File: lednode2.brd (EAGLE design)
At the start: 99.8 x 49.8 mm, 50 parts, among them Q1 AO3402, Q2 AO3402, Q3 AO3402, Q4 AO3402, Q5 AO3402

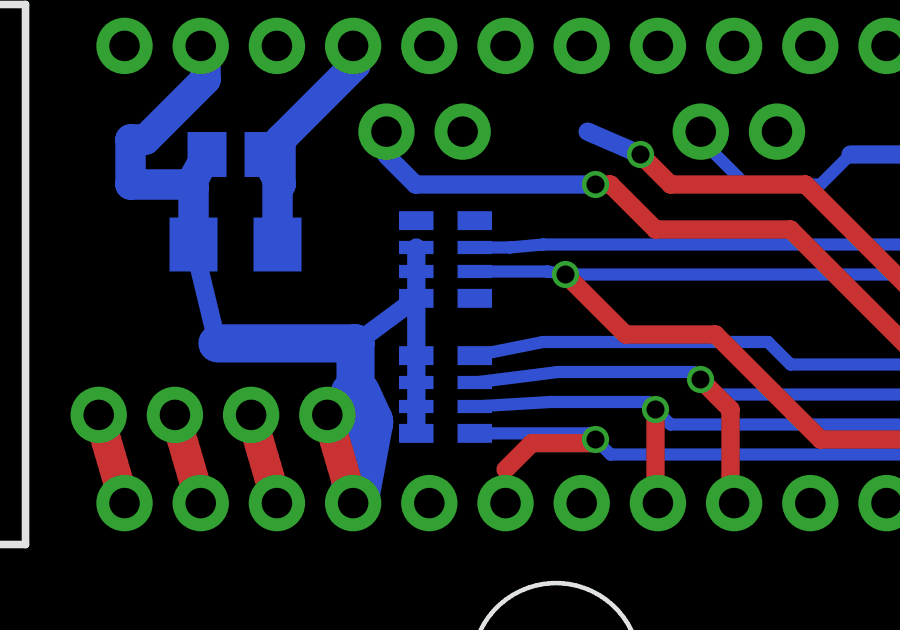
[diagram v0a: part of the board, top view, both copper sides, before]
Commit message: tuning.
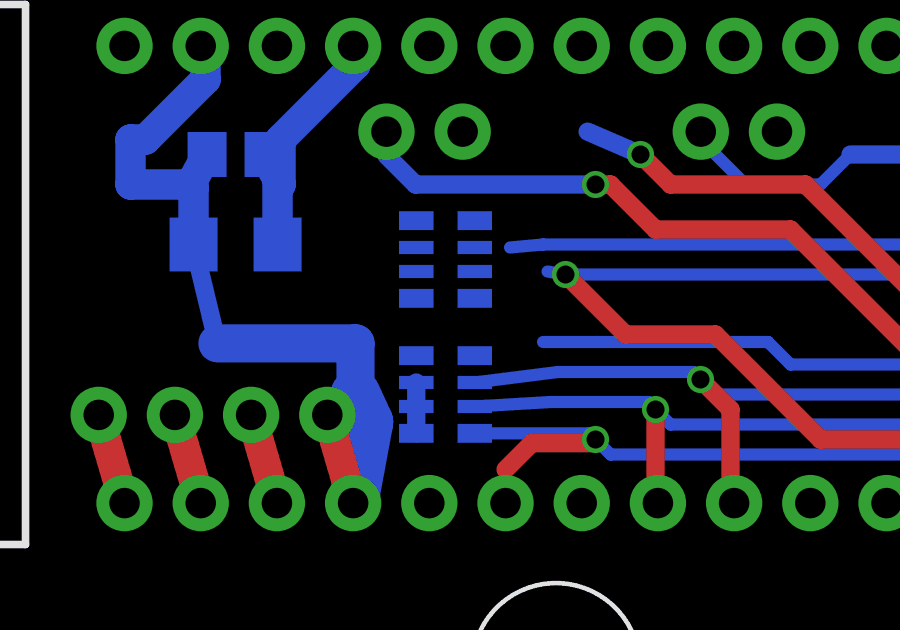
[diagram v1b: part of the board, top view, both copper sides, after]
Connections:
- new net N$12: RN4.3, RN4.4
- new net N$17: RN4.6, RN4.7
- net GND: no longer RN4.3, RN4.4
- net N$13: no longer RN2.5
- net SENSOR1: no longer RN4.8
- net SPOTLIGHT4: now also RN2.5; no longer RN4.7
- net SPOTLIGHT5: now also RN4.8; no longer RN4.6
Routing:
- net GND: track 36.4 -> 29.4 mm
- net SPOTLIGHT4: track 35.5 -> 33.1 mm
- net N$13: track 26.4 -> 24.1 mm
- net SPOTLIGHT5: track 19.6 -> 18.4 mm
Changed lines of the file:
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@@
 <contactref element="LEDS5" pad="3"/>
 <contactref element="Q5" pad="2"/>
-<contactref element="RN4" pad="3"/>
-<contactref element="RN4" pad="2"/>
-<contactref element="RN4" pad="1"/>
-<contactref element="RN2" pad="4"/>
-<wire x1="39.025" y1="28.9" x2="39.025" y2="28.1" width="0.6096" layer="16"/>
-<wire x1="39.025" y1="28.1" x2="39.025" y2="27.205" width="0.6096" layer="16"/>
 <wire x1="39.025" y1="22.705" x2="39.025" y2="23.6" width="0.6096" layer="16"/>
 <wire x1="39.025" y1="23.6" x2="39.025" y2="24.4" width="0.6096" layer="16"/>
-<wire x1="39.025" y1="24.4" x2="39.025" y2="25.295" width="0.6096" layer="16"/>
-<wire x1="39.025" y1="25.295" x2="39.025" y2="27.205" width="0.6096" layer="16"/>
-<wire x1="39.025" y1="27.205" x2="37" y2="25.705" width="0.6096" layer="16"/>
 <wire x1="37" y1="25.705" x2="32.395" y2="25.705" width="1.27" layer="16"/>
 <wire x1="32.395" y1="25.705" x2="31.6" y2="29" width="0.6096" layer="16"/>
@@
 <contactref element="C13" pad="-"/>
 <contactref element="C12" pad="-"/>
-<contactref element="RN4" pad="4"/>
 <contactref element="RN3" pad="4"/>
 <contactref element="C14" pad="-"/>
@@
 <contactref element="C15" pad="-"/>
 <contactref element="L1" pad="3-GND"/>
-<wire x1="70.5" y1="20.27" x2="60.025" y2="30.295" width="0" layer="19" extent="16-16"/>
-<wire x1="39.025" y1="29.795" x2="39.025" y2="28.9" width="0" layer="19" extent="16-16"/>
-<wire x1="12.35" y1="33.55" x2="7.5" y2="36.08" width="0" layer="19" extent="1-1"/>
+<contactref element="RN4" pad="1"/>
+<contactref element="RN2" pad="4"/>
+<contactref element="RN4" pad="2"/>
+<wire x1="73.5" y1="45" x2="86" y2="45" width="0" layer="19" extent="1-1"/>
+<wire x1="76.27" y1="37" x2="73.5" y2="45" width="0" layer="19" extent="1-1"/>
+<wire x1="83.7" y1="31.1" x2="76.27" y2="37" width="0" layer="19" extent="16-16"/>
+<wire x1="80.73" y1="23" x2="83.7" y2="31.1" width="0" layer="19" extent="16-16"/>
+<wire x1="79.55" y1="20" x2="80.73" y2="23" width="0" layer="19" extent="16-16"/>
+<wire x1="84.7" y1="18.1" x2="79.55" y2="20" width="0" layer="19" extent="16-16"/>
+<wire x1="81.1" y1="14.3" x2="84.7" y2="18.1" width="0" layer="19" extent="16-16"/>
+<wire x1="74" y1="19.4" x2="79.55" y2="20" width="0" layer="19" extent="16-16"/>
+<wire x1="70.5" y1="20.27" x2="74" y2="19.4" width="0" layer="19" extent="16-16"/>
+<wire x1="67.1" y1="14.3" x2="70.5" y2="20.27" width="0" layer="19" extent="16-16"/>
+<wire x1="61" y1="45" x2="73.5" y2="45" width="0" layer="19" extent="1-1"/>
+<wire x1="53.1" y1="14.3" x2="67.1" y2="14.3" width="0" layer="19" extent="16-16"/>
+<wire x1="42.41" y1="14.92" x2="53.1" y2="14.3" width="0" layer="19" extent="16-16"/>
+<wire x1="38.92" y1="9" x2="42.41" y2="14.92" width="0" layer="19" extent="1-1"/>
+<wire x1="36.92" y1="20.38" x2="42.41" y2="14.92" width="0" layer="19" extent="16-16"/>
+<wire x1="39.025" y1="22.705" x2="37.42" y2="23.08" width="0" layer="19" extent="16-16"/>
+<wire x1="39.025" y1="25.295" x2="39.025" y2="24.4" width="0" layer="19" extent="16-16"/>
+<wire x1="39.025" y1="27.205" x2="39.025" y2="25.295" width="0" layer="19" extent="16-16"/>
+<wire x1="39.025" y1="28.1" x2="39.025" y2="27.205" width="0" layer="19" extent="16-16"/>
+<wire x1="36" y1="43.05" x2="31.84" y2="35.62" width="0" layer="19" extent="16-16"/>
+<wire x1="40.19" y1="42.73" x2="36" y2="43.05" width="0" layer="19" extent="16-16"/>
+<wire x1="29.73" y1="44" x2="36" y2="43.05" width="0" layer="19" extent="16-16"/>
+<wire x1="20.96" y1="45" x2="29.73" y2="44" width="0" layer="19" extent="1-1"/>
+<wire x1="29.92" y1="9" x2="38.92" y2="9" width="0" layer="19" extent="1-1"/>
+<wire x1="20.92" y1="9" x2="29.92" y2="9" width="0" layer="19" extent="1-1"/>
+<wire x1="11.92" y1="9" x2="20.92" y2="9" width="0" layer="19" extent="1-1"/>
+<wire x1="13.73" y1="16" x2="11.92" y2="9" width="0" layer="19" extent="1-1"/>
+<wire x1="12.9" y1="21" x2="13.73" y2="16" width="0" layer="19" extent="16-16"/>
+<wire x1="13.35" y1="24.5" x2="12.9" y2="21" width="0" layer="19" extent="16-16"/>
+<wire x1="15" y1="27.5" x2="13.35" y2="24.5" width="0" layer="19" extent="16-16"/>
+<wire x1="18" y1="27.5" x2="15" y2="27.5" width="0" layer="19" extent="16-16"/>
+<wire x1="7.5" y1="16.4" x2="13.73" y2="16" width="0" layer="19" extent="1-1"/>
+<wire x1="12.35" y1="33.55" x2="15" y2="27.5" width="0" layer="19" extent="1-16"/>
+<wire x1="7.5" y1="36.08" x2="12.35" y2="33.55" width="0" layer="19" extent="1-1"/>
+<wire x1="20.2606" y1="33.8504" x2="18" y2="27.5" width="0" layer="19" extent="16-16"/>
+<wire x1="60.025" y1="30.295" x2="70.5" y2="20.27" width="0" layer="19" extent="16-16"/>
 </signal>
 <signal name="+5V">
@@
 <signal name="SPOTLIGHT4">
 <contactref element="RN3" pad="2"/>
-<contactref element="RN4" pad="7"/>
 <wire x1="57.24" y1="20.76" x2="55.5" y2="22.5" width="0.6096" layer="1"/>
 <wire x1="55.5" y1="22.5" x2="52.5" y2="22.5" width="0.6096" layer="1"/>
 <wire x1="52.5" y1="22.5" x2="49" y2="26" width="0.6096" layer="1"/>
 <wire x1="49" y1="26" x2="46" y2="26" width="0.6096" layer="1"/>
-<wire x1="40.975" y1="28.1" x2="43.4" y2="28.1" width="0.4064" layer="16"/>
 <wire x1="43.4" y1="28.1" x2="44" y2="28" width="0.4064" layer="16"/>
 <via x="44" y="28" extent="1-16" drill="0.6" shape="octagon"/>
@@
 <wire x1="58" y1="28" x2="44" y2="28" width="0.4064" layer="16"/>
 <contactref element="U$1" pad="12"/>
+<contactref element="RN2" pad="5"/>
 <wire x1="57.24" y1="20.76" x2="57.24" y2="20.38" width="0" layer="19" extent="1-1"/>
+<wire x1="40.975" y1="25.295" x2="43.4" y2="28.1" width="0" layer="19" extent="16-16"/>
 </signal>
 <signal name="LIGHTLEVEL">
@@
 <signal name="SPOTLIGHT5">
 <contactref element="RN3" pad="3"/>
-<contactref element="RN4" pad="6"/>
 <wire x1="57.24" y1="29.24" x2="57" y2="29" width="0.6096" layer="1"/>
 <via x="57" y="29" extent="1-16" drill="0.6" shape="octagon"/>
@@
 <wire x1="60.025" y1="29.4" x2="57.4" y2="29.4" width="0.4064" layer="16"/>
 <wire x1="57.4" y1="29.4" x2="57" y2="29" width="0.4064" layer="16"/>
-<wire x1="40.975" y1="28.9" x2="42.15" y2="28.9" width="0.4064" layer="16"/>
 <wire x1="42.15" y1="28.9" x2="43.25" y2="29" width="0.4064" layer="16"/>
 <contactref element="U$1" pad="13"/>
+<contactref element="RN4" pad="8"/>
 <wire x1="57.4" y1="29.4" x2="57.24" y2="35.62" width="0" layer="19" extent="16-16"/>
+<wire x1="40.975" y1="27.205" x2="42.15" y2="28.9" width="0" layer="19" extent="16-16"/>
 </signal>
 <signal name="SENSOR1">
 <contactref element="IO1" pad="2"/>
-<contactref element="RN4" pad="8"/>
 <contactref element="RN3" pad="1"/>
 <wire x1="60.025" y1="27.705" x2="58.46" y2="45" width="0" layer="19" extent="16-16"/>
-<wire x1="40.975" y1="27.205" x2="60.025" y2="27.705" width="0" layer="19" extent="16-16"/>
 </signal>
 <signal name="N$8">
@@
 <signal name="N$13">
 <contactref element="IO2" pad="2"/>
-<contactref element="RN2" pad="5"/>
 <contactref element="RN1" pad="4"/>
 <wire x1="61.525" y1="24.295" x2="60.705" y2="24.295" width="0.4064" layer="16"/>
 <wire x1="60.705" y1="24.295" x2="60" y2="25" width="0.4064" layer="16"/>
 <wire x1="60" y1="25" x2="51.5" y2="25" width="0.4064" layer="16"/>
-<wire x1="40.975" y1="25.295" x2="43.25" y2="25.75" width="0.4064" layer="16"/>
 <wire x1="43.25" y1="25.75" x2="50.75" y2="25.75" width="0.4064" layer="16"/>
 <wire x1="50.75" y1="25.75" x2="51.5" y2="25" width="0.4064" layer="16"/>
@@
 <wire x1="15.65" y1="33.55" x2="39.46" y2="35.62" width="0" layer="19" extent="1-1"/>
 </signal>
+<signal name="N$12">
+<contactref element="RN4" pad="4"/>
+<contactref element="RN4" pad="3"/>
+<wire x1="39.025" y1="28.9" x2="39.025" y2="29.795" width="0" layer="19" extent="16-16"/>
+</signal>
+<signal name="N$17">
+<contactref element="RN4" pad="6"/>
+<contactref element="RN4" pad="7"/>
+<wire x1="40.975" y1="28.1" x2="40.975" y2="28.9" width="0" layer="19" extent="16-16"/>
+</signal>
 </signals>
